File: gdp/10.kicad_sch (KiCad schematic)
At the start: 8 parts, among them IC46 2732, IC47 HM6116, IC50 SCB2675

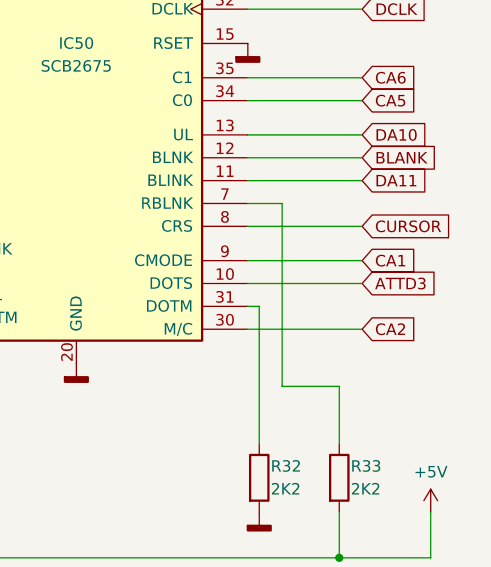
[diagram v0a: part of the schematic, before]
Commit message: Fixes "CA0" issue in schematics
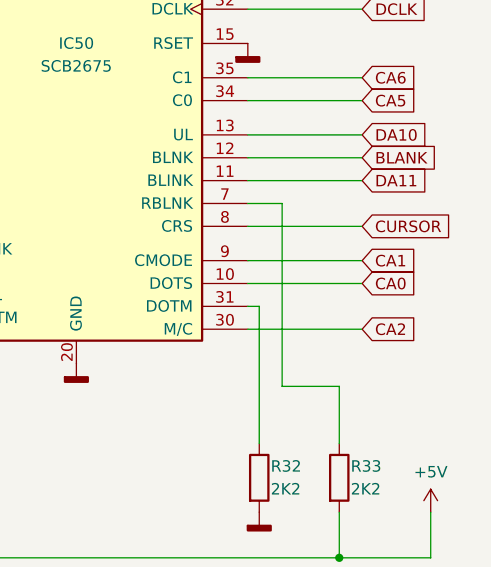
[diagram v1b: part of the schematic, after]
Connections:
- net ATTD3 renamed CA0
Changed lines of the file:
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@@
 (kicad_sch
-	(version 20231120)
+	(version 20250114)
 	(generator "eeschema")
-	(generator_version "8.0")
+	(generator_version "9.0")
 	(paper "A4")
 	(title_block
@@
 		)
 	)
-	(global_label "ATTD3"
+	(global_label "CA0"
 		(shape input)
 		(at 238.76 109.22 0)
@@
 		)
 		(property "Intersheetrefs" "${INTERSHEET_REFS}"
-			(at 247.2485 109.22 0)
+			(at 245.3133 109.22 0)
 			(effects
 				(font
